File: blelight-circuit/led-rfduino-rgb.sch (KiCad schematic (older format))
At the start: 16 parts, among them P1 POWER_REGULATOR, Q1 N_CHAN_MOSFET, Q2 N_CHAN_MOSFET, Q3 N_CHAN_MOSFET

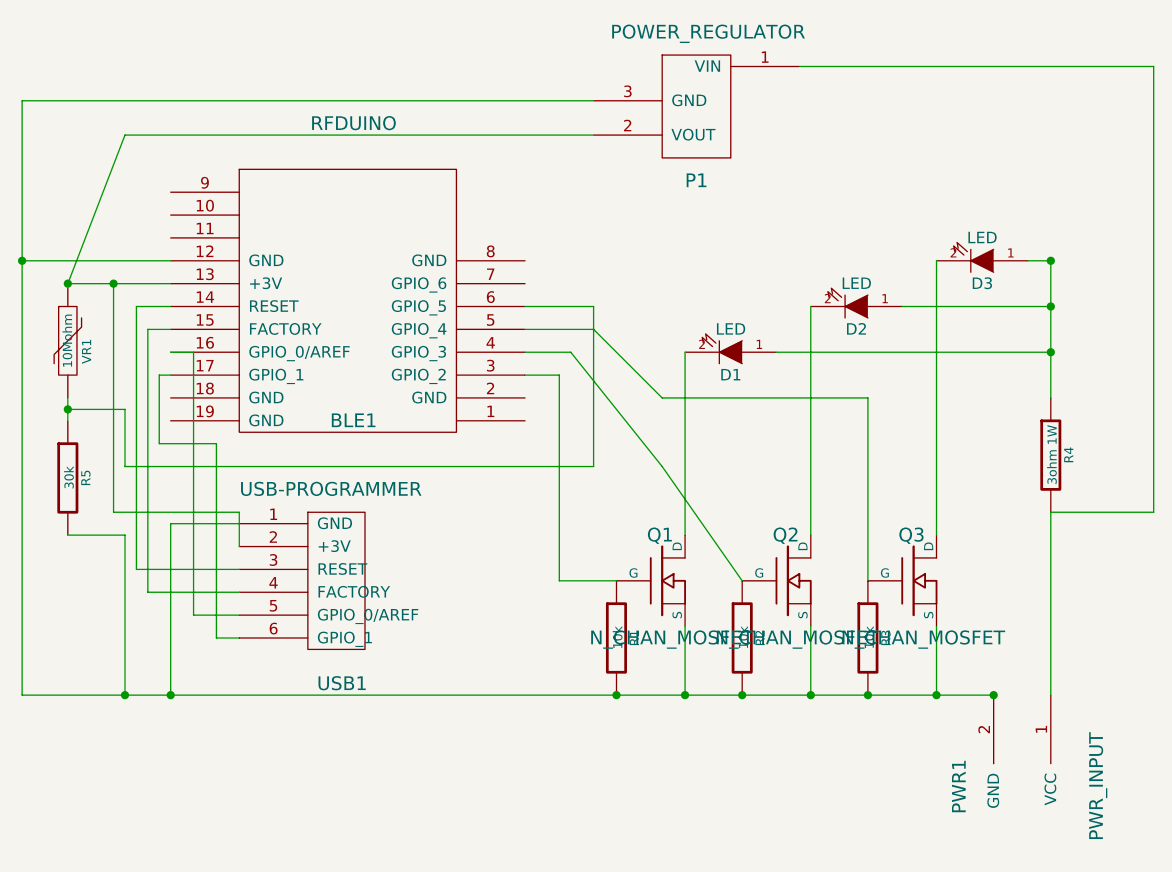
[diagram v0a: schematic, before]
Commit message: lightserver working
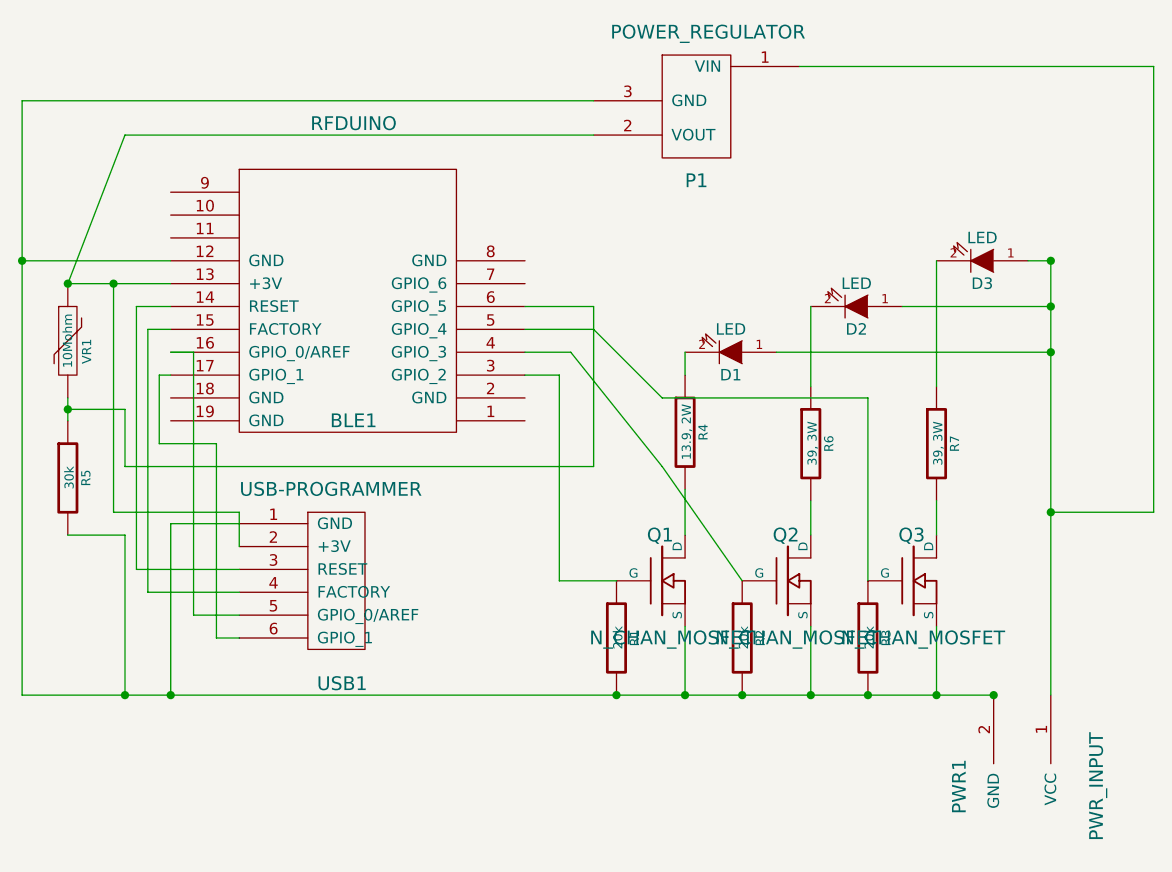
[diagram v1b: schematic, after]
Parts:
- added R6, R7: 39, 3W, ~, symbol R
- R1, R2, R3: value 10k -> 20k
- R4: value 3ohm 1W -> 13.9, 2W
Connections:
- net at D1.1 (A), D2.1 (A), D3.1 (A): now also P1.1 (VIN), PWR1.1 (VCC); no longer R4.1
- net at D3.2 (K): now also R7.1; no longer Q3.3 (D)
- net at D2.2 (K): now also R6.1; no longer Q2.3 (D)
- net at D1.2 (K): now also R4.1; no longer Q1.3 (D)
- new net: Q1.3 (D), R4.2
- new net: Q2.3 (D), R6.2
- new net: Q3.3 (D), R7.2
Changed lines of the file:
@@
 Sheet 1 1
 Title ""
-Date "24 feb 2015"
+Date "21 mar 2015"
 Rev ""
 Comp ""
@@
 Comment4 ""
 $EndDescr
-$Comp
-L R R4
-U 1 1 54E9181E
-P 6300 2250
-F 0 "R4" V 6380 2250 40  0000 C CNN
-F 1 "3ohm 1W" V 6307 2251 40  0000 C CNN
-F 2 "~" V 6230 2250 30  0000 C CNN
-F 3 "~" H 6300 2250 30  0000 C CNN
-	1    6300 2250
-	1    0    0    -1
-$EndComp
 $Comp
 L RFDUINO BLE1
@@
 P 4400 3050
 F 0 "R1" V 4480 3050 40  0000 C CNN
-F 1 "10k" V 4407 3051 40  0000 C CNN
+F 1 "20k" V 4407 3051 40  0000 C CNN
 F 2 "~" V 4330 3050 30  0000 C CNN
 F 3 "~" H 4400 3050 30  0000 C CNN
@@
 P 4950 3050
 F 0 "R2" V 5030 3050 40  0000 C CNN
-F 1 "10k" V 4957 3051 40  0000 C CNN
+F 1 "20k" V 4957 3051 40  0000 C CNN
 F 2 "~" V 4880 3050 30  0000 C CNN
 F 3 "~" H 4950 3050 30  0000 C CNN
@@
 P 5500 3050
 F 0 "R3" V 5580 3050 40  0000 C CNN
-F 1 "10k" V 5507 3051 40  0000 C CNN
+F 1 "20k" V 5507 3051 40  0000 C CNN
 F 2 "~" V 5430 3050 30  0000 C CNN
 F 3 "~" H 5500 3050 30  0000 C CNN
@@
 $EndComp
 Wire Wire Line
-	1800 700  1800 3300
-Wire Wire Line
-	1800 3300 6050 3300
+	1800 700  1800 1400
+Wire Wire Line
+	1800 1400 1800 3300
+Wire Wire Line
+	1800 3300 2250 3300
+Wire Wire Line
+	2250 3300 2450 3300
+Wire Wire Line
+	2450 3300 4400 3300
+Wire Wire Line
+	4400 3300 4700 3300
+Wire Wire Line
+	4700 3300 4950 3300
+Wire Wire Line
+	4950 3300 5250 3300
+Wire Wire Line
+	5250 3300 5500 3300
+Wire Wire Line
+	5500 3300 5800 3300
+Wire Wire Line
+	5800 3300 6050 3300
 Connection ~ 6050 3300
 Wire Wire Line
-	6300 3300 6300 2500
+	6300 1400 6300 1600
+Wire Wire Line
+	6300 1600 6300 1800
+Wire Wire Line
+	6300 1800 6300 2500
+Wire Wire Line
+	6300 2500 6300 3300
 $Comp
 L LED D3
@@
 Connection ~ 6300 1800
 Wire Wire Line
-	4700 1800 4700 2600
-Wire Wire Line
-	5250 1600 5250 2600
-Wire Wire Line
-	5800 1400 5800 2600
-Wire Wire Line
 	5800 3000 5800 3300
 Connection ~ 5800 3300
@@
 Connection ~ 1800 1400
 Wire Wire Line
-	2000 1500 2450 1500
+	2000 1500 2200 1500
+Wire Wire Line
+	2200 1500 2450 1500
 Connection ~ 2000 1500
 Wire Wire Line
 	2250 2600 2000 2600
 Wire Wire Line
-	2000 2000 2000 2100
+	2000 2000 2000 2050
+Wire Wire Line
+	2000 2050 2000 2100
 Wire Wire Line
 	2000 1500 2250 850
@@
 Wire Wire Line
 	6750 2500 6300 2500
-Wire Wire Line
-	6300 1400 6300 2000
 Connection ~ 5500 3300
 Connection ~ 4950 3300
@@
 Wire Wire Line
 	2400 1900 2450 1900
+Connection ~ 6300 2500
+$Comp
+L R R7
+U 1 1 550CBB60
+P 5800 2200
+F 0 "R7" V 5880 2200 40  0000 C CNN
+F 1 "39, 3W" V 5807 2201 40  0000 C CNN
+F 2 "~" V 5730 2200 30  0000 C CNN
+F 3 "~" H 5800 2200 30  0000 C CNN
+	1    5800 2200
+	1    0    0    -1
+$EndComp
+Wire Wire Line
+	5800 2600 5800 2450
+Wire Wire Line
+	5800 1950 5800 1400
+$Comp
+L R R6
+U 1 1 550CBC4B
+P 5250 2200
+F 0 "R6" V 5330 2200 40  0000 C CNN
+F 1 "39, 3W" V 5257 2201 40  0000 C CNN
+F 2 "~" V 5180 2200 30  0000 C CNN
+F 3 "~" H 5250 2200 30  0000 C CNN
+	1    5250 2200
+	1    0    0    -1
+$EndComp
+Wire Wire Line
+	5250 2600 5250 2450
+Wire Wire Line
+	5250 1950 5250 1600
+$Comp
+L R R4
+U 1 1 550CBCFB
+P 4700 2150
+F 0 "R4" V 4780 2150 40  0000 C CNN
+F 1 "13.9, 2W" V 4707 2151 40  0000 C CNN
+F 2 "~" V 4630 2150 30  0000 C CNN
+F 3 "~" H 4700 2150 30  0000 C CNN
+	1    4700 2150
+	1    0    0    -1
+$EndComp
+Wire Wire Line
+	4700 1800 4700 1900
+Wire Wire Line
+	4700 2400 4700 2600
 $EndSCHEMATC
